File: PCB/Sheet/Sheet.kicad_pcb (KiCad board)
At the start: 2 copper layers, 54.8 x 47.7 mm, 30 parts, among them IC1 ADXL33X, U1 MCP9700Ax-ELT, U2 MCP2562-E-MF, U3 ATtiny1616-M, U5 CD74HC4067SM, U6 MCP2515-xST, U7 DRV5055A1xDBZxQ1, U8 DRV5055A1xDBZxQ1

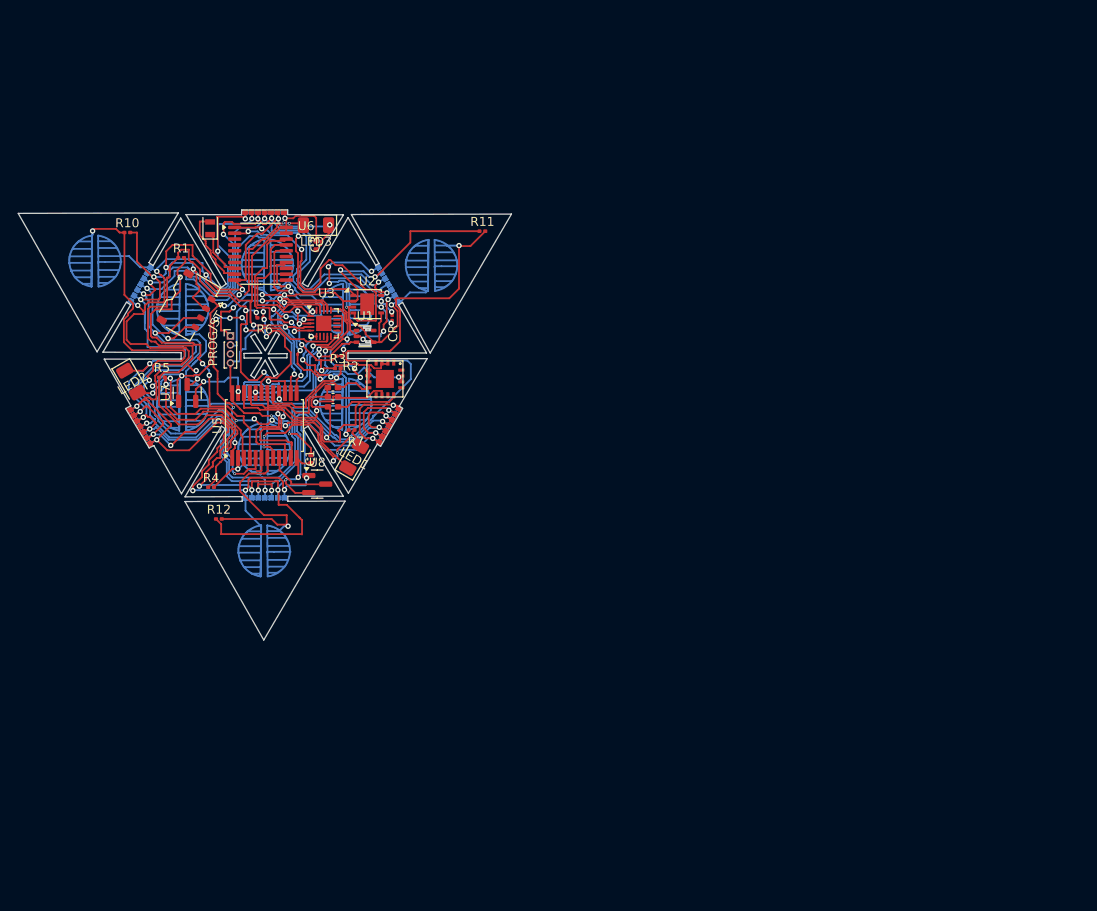
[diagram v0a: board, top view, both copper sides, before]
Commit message: reorg
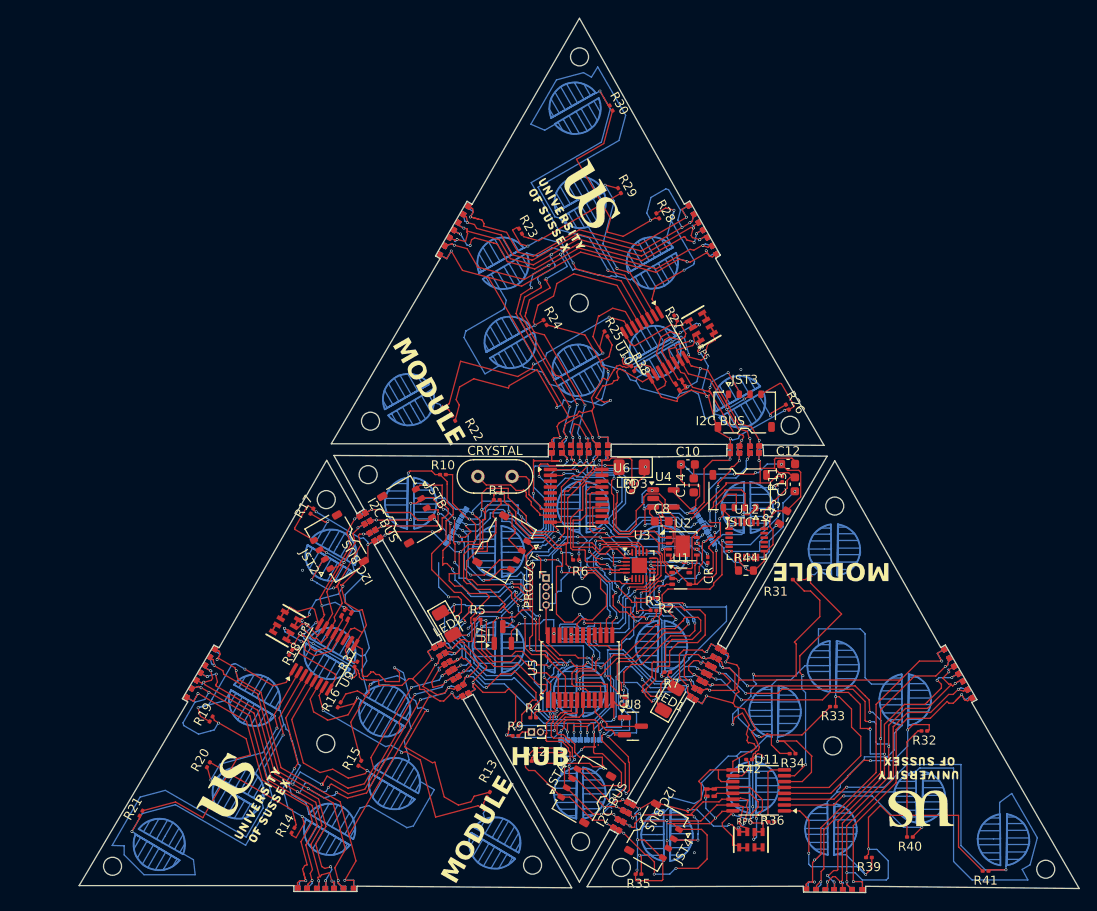
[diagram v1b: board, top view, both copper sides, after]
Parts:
- removed C1A, C2A, C3A: C_0402_1005Metric_Pad0.74x0.62mm_HandSolder, Capacitor_SMD:C_0402_1005Metric_Pad0.74x0.62mm_HandSolder
- removed IC1: ADXL33X, 16LCSP
- removed crystal: Crystal_SMD_2012-2Pin_2.0x1.2mm, Crystal:Crystal_SMD_2012-2Pin_2.0x1.2mm
- added C10: 0.1uF, Capacitor_SMD:C_0603_1608Metric, F.Cu at (218.0, 103.4)
- added C12: 0.1uF, Capacitor_SMD:C_0603_1608Metric, F.Cu at (229.1, 103.4)
- added C13: 0.1uF, Capacitor_SMD:C_0603_1608Metric, F.Cu at (229.9, 105.6)
- added C14: 220pF, Capacitor_SMD:C_0603_1608Metric, F.Cu at (218.6, 105.8)
- added C8: 4.7uF, Capacitor_SMD:C_0603_1608Metric, F.Cu at (215.1, 109.8)
- added CRYSTAL: Crystal_HC52-6mm_Vertical, Crystal:Crystal_HC52-6mm_Vertical, F.Cu at (194.7, 104.8)
- added G***: LOGO, LOGO, F.Cu at (168.5, 140.2)
- added G***1: LOGO, LOGO, F.Cu at (205.6, 74.6)
- added G***2: LOGO, LOGO, F.Cu at (243.7, 139.8)
- added JST2: JST_ACH_BM04B-ACHSS-A-GAN-ETF_1x04-1MP_P1.20mm_Vertical, Connector_JST:JST_ACH_BM04B-ACHSS-A-GAN-ETF_1x04-1MP_P1.20mm_Vertical, F.Cu at (179.0, 112.5)
- added JST3: JST_ACH_BM04B-ACHSS-A-GAN-ETF_1x04-1MP_P1.20mm_Vertical, Connector_JST:JST_ACH_BM04B-ACHSS-A-GAN-ETF_1x04-1MP_P1.20mm_Vertical, F.Cu at (224.3, 97.5)
- added JST4: JST_ACH_BM04B-ACHSS-A-GAN-ETF_1x04-1MP_P1.20mm_Vertical, Connector_JST:JST_ACH_BM04B-ACHSS-A-GAN-ETF_1x04-1MP_P1.20mm_Vertical, F.Cu at (214.5, 144.6)
- added JSTA: JST_ACH_BM04B-ACHSS-A-GAN-ETF_1x04-1MP_P1.20mm_Vertical, Connector_JST:JST_ACH_BM04B-ACHSS-A-GAN-ETF_1x04-1MP_P1.20mm_Vertical, F.Cu at (206.5, 139.8)
- added JSTB: JST_ACH_BM04B-ACHSS-A-GAN-ETF_1x04-1MP_P1.20mm_Vertical, Connector_JST:JST_ACH_BM04B-ACHSS-A-GAN-ETF_1x04-1MP_P1.20mm_Vertical, F.Cu at (187.1, 108.7)
- added JSTC: JST_ACH_BM04B-ACHSS-A-GAN-ETF_1x04-1MP_P1.20mm_Vertical, Connector_JST:JST_ACH_BM04B-ACHSS-A-GAN-ETF_1x04-1MP_P1.20mm_Vertical, F.Cu at (223.7, 106.4)
- added P1: C_0201_0603Metric_Pad0.64x0.40mm_HandSolder, Capacitor_SMD:C_0201_0603Metric_Pad0.64x0.40mm_HandSolder, F.Cu at (179.7, 119.9)
- added P1: C_0201_0603Metric_Pad0.64x0.40mm_HandSolder, Capacitor_SMD:C_0201_0603Metric_Pad0.64x0.40mm_HandSolder, F.Cu at (180.4, 120.3)
- added P2: C_0201_0603Metric_Pad0.64x0.40mm_HandSolder, Capacitor_SMD:C_0201_0603Metric_Pad0.64x0.40mm_HandSolder, F.Cu at (216.9, 94.9)
- added P3: C_0201_0603Metric_Pad0.64x0.40mm_HandSolder, Capacitor_SMD:C_0201_0603Metric_Pad0.64x0.40mm_HandSolder, F.Cu at (217.5, 94.5)
- added P4: C_0201_0603Metric_Pad0.64x0.40mm_HandSolder, Capacitor_SMD:C_0201_0603Metric_Pad0.64x0.40mm_HandSolder, F.Cu at (220.5, 139.5)
- added P5: C_0201_0603Metric_Pad0.64x0.40mm_HandSolder, Capacitor_SMD:C_0201_0603Metric_Pad0.64x0.40mm_HandSolder, F.Cu at (220.5, 140.3)
- added R13: R, Resistor_SMD:R_0201_0603Metric, F.Cu at (195.8, 140.1)
- added R14: R, Resistor_SMD:R_0201_0603Metric, F.Cu at (174.2, 144.1)
- added R15: R, Resistor_SMD:R_0201_0603Metric, F.Cu at (181.6, 136.6)
- added R16: R, Resistor_SMD:R_0201_0603Metric, F.Cu at (179.3, 130.1)
- added R17: R, Resistor_SMD:R_0201_0603Metric, F.Cu at (176.3, 108.6)
- added R18: R, Resistor_SMD:R_0201_0603Metric, F.Cu at (173.9, 124.3)
- added R19: R, Resistor_SMD:R_0201_0603Metric, F.Cu at (165.1, 131.7)
- added R20: R, Resistor_SMD:R_0201_0603Metric, F.Cu at (164.8, 136.8)
- added R21: R, Resistor_SMD:R_0201_0603Metric, F.Cu at (157.3, 142.2)
- added R22: R, Resistor_SMD:R_0201_0603Metric, F.Cu at (192.0, 98.3)
- added R23: R, Resistor_SMD:R_0201_0603Metric, F.Cu at (199.4, 77.6)
- added R24: R, Resistor_SMD:R_0201_0603Metric, F.Cu at (202.1, 87.7)
- added R25: R, Resistor_SMD:R_0201_0603Metric, F.Cu at (208.9, 89.0)
- added R26: R, Resistor_SMD:R_0201_0603Metric, F.Cu at (229.0, 97.1)
- added R27: R, Resistor_SMD:R_0201_0603Metric, F.Cu at (216.6, 87.2)
- added R28: R, Resistor_SMD:R_0201_0603Metric, F.Cu at (214.6, 75.9)
- added R29: R, Resistor_SMD:R_0201_0603Metric, F.Cu at (210.4, 73.0)
- added R30: R, Resistor_SMD:R_0201_0603Metric, F.Cu at (209.5, 63.9)
- added R31: R, Resistor_SMD:R_0201_0603Metric, F.Cu at (230.0, 116.2)
- added R32: R, Resistor_SMD:R_0201_0603Metric, F.Cu at (244.2, 133.0)
- added R33: R, Resistor_SMD:R_0201_0603Metric, F.Cu at (234.1, 130.3)
- added R34: R, Resistor_SMD:R_0201_0603Metric, F.Cu at (229.6, 135.6)
- added R35: R, Resistor_SMD:R_0201_0603Metric, F.Cu at (212.5, 148.9)
- added R36: R, Resistor_SMD:R_0201_0603Metric, F.Cu at (227.3, 143.1)
- added R37: R, Resistor_SMD:R_0201_0603Metric, F.Cu at (181.1, 125.6)
- added R38: R, Resistor_SMD:R_0201_0603Metric, F.Cu at (211.9, 92.8)
- added R39: R, Resistor_SMD:R_0201_0603Metric, F.Cu at (238.1, 147.1)
- added R40: R, Resistor_SMD:R_0201_0603Metric, F.Cu at (242.6, 144.8)
- added R41: R, Resistor_SMD:R_0201_0603Metric, F.Cu at (251.0, 148.6)
- added R42: R, Resistor_SMD:R_0201_0603Metric, F.Cu at (224.8, 136.2)
- added R43: 4.7k, Resistor_SMD:R_0603_1608Metric, F.Cu at (228.6, 109.3)
- added R44: 4.7k, Resistor_SMD:R_0603_1608Metric, F.Cu at (224.4, 115.2)
- added R9: R9, Resistor_SMD:R_0201_0603Metric, F.Cu at (198.8, 133.6)
- added REF**: PinHeader_1x02_P1.00mm_Vertical, Connector_PinHeader_1.00mm:PinHeader_1x02_P1.00mm_Vertical, F.Cu at (200.6, 133.2)
- added RP4: 10K Pack, RESPACK_4X0603, F.Cu at (173.3, 121.3)
- added RP5: 10K Pack, RESPACK_4X0603, F.Cu at (219.5, 88.2)
- added RP6: 10K Pack, RESPACK_4X0603, F.Cu at (225.0, 145.1)
- added U10: ADS7830, Package_SO:TSSOP-16_4.4x5mm_P0.65mm, F.Cu at (214.3, 90.2)
- added U11: ADS7830, Package_SO:TSSOP-16_4.4x5mm_P0.65mm, F.Cu at (225.8, 139.6)
- added U12: MPU-6050, Sensor_Motion:InvenSense_QFN-24_4x4mm_P0.5mm, F.Cu at (224.5, 111.8)
- added U4: AP2112K-3.3, Package_TO_SOT_SMD:SOT-23-5, F.Cu at (215.3, 107.2)
- added U9: ADS7830, Package_SO:TSSOP-16_4.4x5mm_P0.65mm, F.Cu at (177.6, 124.8)
- C1, C3: value C_0402_1005Metric -> C
- R1, R10, R11, R12, R2, R3, R4, R5, R6, R7: value R_0201_0603Metric -> R
- moved R10 44.2 mm to (190.8, 104.6)
- moved R5 44.2 mm to (194.6, 120.7)
- moved R7 44.2 mm to (215.7, 126.5)
- moved U3 44.2 mm to (212.6, 114.7)
- moved C3 44.2 mm to (211.8, 106.0)
- moved CR 44.2 mm to (220.2, 114.0)
- moved JST 44.2 mm to (197.6, 112.6)
- moved LED1 44.2 mm to (216.0, 129.5)
- moved LED2 44.2 mm to (191.2, 121.1)
- moved LED3 44.2 mm to (211.8, 103.8)
- moved PROG 44.2 mm to (202.2, 116.0)
- moved R1 44.2 mm to (196.8, 107.4)
- moved R12 44.2 mm to (201.0, 136.4)
- moved R2 44.2 mm to (214.3, 118.3)
- moved R3 44.2 mm to (214.2, 119.7)
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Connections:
- C1 pad 1: (no net) -> Net-(MK1--)
- C1 pad 2: (no net) -> Net-(U1-V_{DD})
- C3 pad 1: (no net) -> Net-(U1-V_{DD})
- C3 pad 2: (no net) -> Net-(MK1--)
- R1 pad 1: (no net) -> Net-(MK1--)
- R1 pad 2: (no net) -> Net-(U5-I5)
- R10 pad 1: (no net) -> Net-(MK1--)
- R10 pad 2: (no net) -> Net-(U5-I4)
- R11 pad 1: (no net) -> Net-(MK1--)
- R11 pad 2: (no net) -> Net-(U5-I2)
- R12 pad 1: (no net) -> Net-(MK1--)
- R12 pad 2: (no net) -> Net-(U5-I1)
- R2 pad 1: (no net) -> Net-(MK1--)
- R2 pad 2: (no net) -> Net-(U5-I15)
- R3 pad 1: (no net) -> Net-(MK1--)
- R3 pad 2: (no net) -> Net-(U5-I14)
- R4 pad 1: (no net) -> Net-(MK1--)
- R4 pad 2: (no net) -> Net-(U5-I7)
- R5 pad 1: (no net) -> Net-(MK1--)
- R5 pad 2: (no net) -> Net-(U5-I6)
- R6 pad 1: (no net) -> Net-(MK1--)
- R6 pad 2: (no net) -> Net-(U5-I12)
- R7 pad 1: (no net) -> Net-(U3-PA5)
- R7 pad 2: (no net) -> Net-(D1-A)
- U1 pad 1: (no net) -> unconnected-(U1-NC-Pad1)
- U1 pad 2: (no net) -> Net-(D3-K)
- U1 pad 3: (no net) -> Net-(U1-V_{OUT})
- U1 pad 4: (no net) -> Net-(U1-V_{DD})
- U1 pad 5: (no net) -> unconnected-(U1-NC-Pad5)
- U2 pad 1: (no net) -> Net-(U2-TXD)
- U2 pad 2: (no net) -> Net-(MK1--)
- U2 pad 3: (no net) -> Net-(U1-V_{DD})
- U2 pad 4: (no net) -> Net-(U2-RXD)
- U2 pad 5: (no net) -> Net-(U1-V_{DD})
- U2 pad 6: (no net) -> Net-(U2-CANL)
- U2 pad 7: (no net) -> Net-(U2-CANH)
- U2 pad 8: (no net) -> unconnected-(U2-SHDN-Pad8)
- U2 pad 9: (no net) -> unconnected-(U2-PAD-Pad9)
- U3 pad 1: (no net) -> Net-(U3-PA2)
- U3 pad 10: (no net) -> unconnected-(U3-PB4-Pad10)
- U3 pad 11: (no net) -> unconnected-(U3-PB3-Pad11)
- U3 pad 12: (no net) -> unconnected-(U3-PB2-Pad12)
- U3 pad 13: (no net) -> Net-(U10-SDA)
- U3 pad 14: (no net) -> Net-(U10-SCL)
- U3 pad 15: (no net) -> Net-(U3-PC0)
- U3 pad 16: (no net) -> Net-(U3-PC1)
- U3 pad 17: (no net) -> Net-(U3-PC2)
- U3 pad 18: (no net) -> Net-(U3-PC3)
- U3 pad 19: (no net) -> unconnected-(U3-~{RESET}/PA0-Pad19)
- U3 pad 2: (no net) -> Net-(U3-PA3)
- U3 pad 20: (no net) -> Net-(U3-PA1)
- U3 pad 21: (no net) -> Net-(D3-K)
- U3 pad 3: (no net) -> Net-(D3-K)
- U3 pad 4: (no net) -> Net-(U3-VCC)
- U3 pad 5: (no net) -> Net-(U3-PA4)
- U3 pad 6: (no net) -> Net-(U3-PA5)
- U3 pad 7: (no net) -> unconnected-(U3-PA6-Pad7)
- U3 pad 8: (no net) -> unconnected-(U3-PA7-Pad8)
- U3 pad 9: (no net) -> Net-(U3-PB5)
- U5 pad 1: (no net) -> Net-(U3-PB5)
- U5 pad 10: (no net) -> Net-(U3-PC0)
- U5 pad 11: (no net) -> Net-(U3-PC1)
- U5 pad 12: (no net) -> Net-(MK1--)
- U5 pad 13: (no net) -> Net-(U3-PC3)
- U5 pad 14: (no net) -> Net-(U3-PC2)
- U5 pad 15: (no net) -> Net-(MK1--)
- U5 pad 16: (no net) -> Net-(U5-I15)
- U5 pad 17: (no net) -> Net-(U5-I14)
- U5 pad 18: (no net) -> unconnected-(U5-I13-Pad18)
- U5 pad 19: (no net) -> Net-(U5-I12)
- U5 pad 2: (no net) -> Net-(U5-I7)
- U5 pad 20: (no net) -> Net-(U1-V_{OUT})
- U5 pad 21: (no net) -> unconnected-(U5-I10-Pad21)
- U5 pad 22: (no net) -> unconnected-(U5-I9-Pad22)
- U5 pad 23: (no net) -> Net-(U5-I8)
- U5 pad 24: (no net) -> Net-(U1-V_{DD})
- U5 pad 3: (no net) -> Net-(U5-I6)
- U5 pad 4: (no net) -> Net-(U5-I5)
- U5 pad 5: (no net) -> Net-(U5-I4)
- U5 pad 6: (no net) -> Net-(MK1-+)
- U5 pad 7: (no net) -> Net-(U5-I2)
- U5 pad 8: (no net) -> Net-(U5-I1)
- U5 pad 9: (no net) -> Net-(U5-I0)
- U6 pad 1: (no net) -> Net-(U2-TXD)
- U6 pad 10: (no net) -> Net-(MK1--)
- U6 pad 11: (no net) -> unconnected-(U6-~{RX1BF}-Pad11)
- U6 pad 12: (no net) -> unconnected-(U6-~{RX0BF}-Pad12)
- U6 pad 13: (no net) -> unconnected-(U6-~{INT}-Pad13)
- U6 pad 14: (no net) -> Net-(U3-PA3)
- U6 pad 15: (no net) -> unconnected-(U6-NC-Pad15)
- U6 pad 16: (no net) -> Net-(U3-PA1)
- U6 pad 17: (no net) -> Net-(U3-PA2)
- U6 pad 18: (no net) -> Net-(U3-PA4)
- U6 pad 19: (no net) -> Net-(U1-V_{DD})
- U6 pad 2: (no net) -> Net-(U2-RXD)
- U6 pad 20: (no net) -> Net-(U1-V_{DD})
- U6 pad 3: (no net) -> unconnected-(U6-CLKOUT/SOF-Pad3)
- U6 pad 4: (no net) -> unconnected-(U6-~{TX0RTS}-Pad4)
- U6 pad 5: (no net) -> unconnected-(U6-~{TX1RTS}-Pad5)
- U6 pad 6: (no net) -> unconnected-(U6-NC-Pad6)
- U6 pad 7: (no net) -> unconnected-(U6-~{TX2RTS}-Pad7)
- U6 pad 8: (no net) -> Net-(U6-OSC2)
- U6 pad 9: (no net) -> Net-(U6-OSC1)
- U7 pad 1: (no net) -> Net-(U1-V_{DD})
- U7 pad 2: (no net) -> Net-(U5-I8)
- U7 pad 3: (no net) -> Net-(MK1--)
- U8 pad 1: (no net) -> Net-(U1-V_{DD})
- U8 pad 2: (no net) -> Net-(U5-I0)
- U8 pad 3: (no net) -> Net-(MK1--)
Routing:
- net Net-(MK1--): track 0.00 -> 1216.2 mm, vias 0 -> 64
- net Net-(U1-V_{DD}): track 0.00 -> 1055.6 mm, vias 0 -> 120
- net (no net): track 1925.3 -> 1211.9 mm, vias 163 -> 74
- net Net-(U2-CANL): track 0.00 -> 326.2 mm, vias 0 -> 32
- net Net-(U10-SCL): track 0.00 -> 189.5 mm, vias 0 -> 27
- net Net-(U9-CH0): track 0.00 -> 166.8 mm, vias 0 -> 9
- net Net-(U2-CANH): track 0.00 -> 159.2 mm, vias 0 -> 21
- net Net-(U9-CH2): track 0.00 -> 117.3 mm, vias 0 -> 6
- net Net-(U10-SDA): track 0.00 -> 110.9 mm, vias 0 -> 9
- net Net-(U5-I5): track 0.00 -> 103.4 mm, vias 0 -> 9
- net Net-(U9-CH1): track 0.00 -> 90.0 mm, vias 0 -> 6
- net Net-(U9-CH4): track 0.00 -> 77.7 mm, vias 0 -> 3
- net Net-(U10-CH0): track 0.00 -> 75.5 mm, vias 0 -> 3
- net Net-(U5-I7): track 0.00 -> 74.1 mm, vias 0 -> 13
- net Net-(U9-CH3): track 0.00 -> 65.1 mm, vias 0 -> 6
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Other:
- board size 54.8 x 47.7 mm -> 111 x 97.1 mm
- board text added: "HUB"
- board text added: "I2C BUS"
- board text added: "MODULE"
